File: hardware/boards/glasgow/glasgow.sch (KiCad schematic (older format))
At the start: 93 parts, among them J1 USB_B_Micro, U1 CY7C68013A-56LTX, U15 TPD3S014, U2 CAT24M01W, U3 CAT24C256W, U30 ICE40HX8K-BG121, U34 ATECC508A, U36 TLV73312PQDRVRQ1, U7 LM3880MF-1AF, U8 TLV75533PDRVR, Y1 24M

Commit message: revC2: added output files
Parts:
- removed J1: USB_B_Micro, Connector_USB:USB_Micro-B_Molex_47346-0001, symbol Connector:USB_B_Micro
- added J1: USB_C_Plug_USB2.0, Glasgow:USB-C_16Pin, symbol Connector:USB_C_Plug_USB2.0
- added R52, R53: 5k1, Resistor_SMD:R_0402_1005Metric, symbol Device:R
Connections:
- wire segments 364 -> 371
- no-connect marks 8 -> 7
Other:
- moved on the sheet: C13, FB1, R1, R2, R3, TP13, TP14, TP15, TP16, TP4, TP5

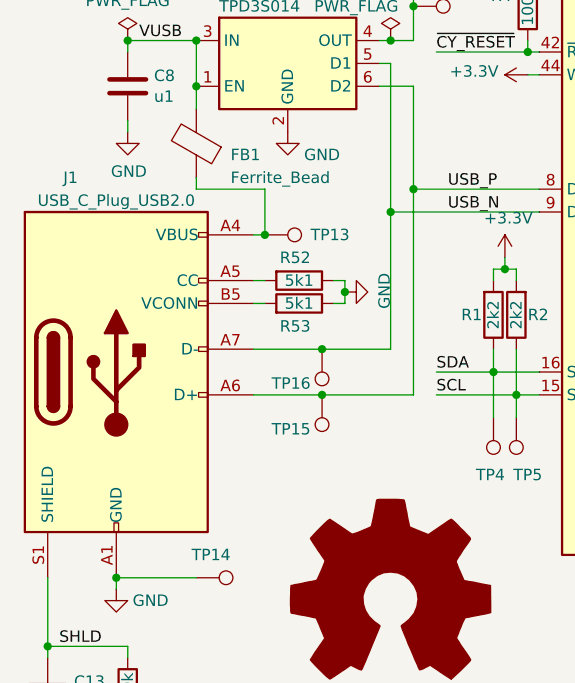
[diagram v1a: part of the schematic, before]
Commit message: added revC1 otter edition gerber
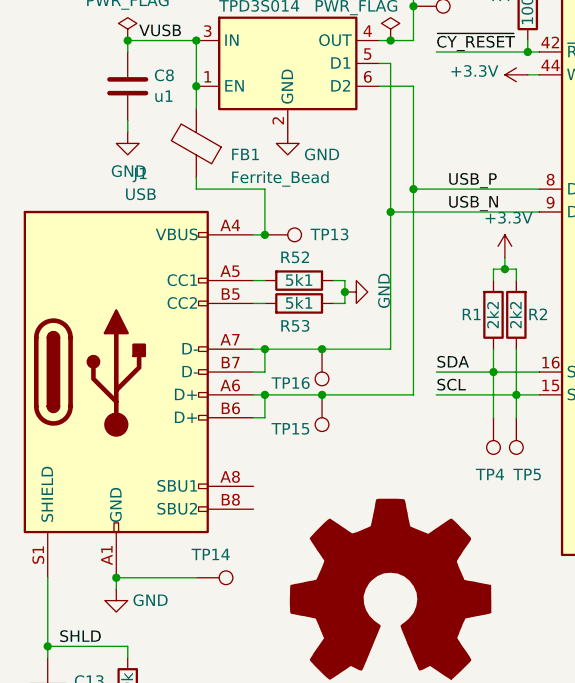
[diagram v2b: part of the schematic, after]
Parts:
- removed J1: USB_C_Plug_USB2.0, Glasgow:USB-C_16Pin, symbol Connector:USB_C_Plug_USB2.0
- added J1: USB, otter:USB-C 16Pin, symbol Connector:USB_C_Receptacle_USB2.0
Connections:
- net GND: now also J1.A1 (GND), J1.A12 (GND), J1.B1 (GND), J1.B12 (GND)
- net SHLD: now also J1.S1 (SHIELD)
- net USB_N: now also J1.A7 (D-), J1.B7 (D-)
- net USB_P: now also J1.A6 (D+), J1.B6 (D+)
- net at FB1.1, TP13.1: now also J1.A4 (VBUS), J1.A9 (VBUS), J1.B4 (VBUS), J1.B9 (VBUS)
- net at R52.2: now also J1.A5 (CC1)
- net at R53.2: now also J1.B5 (CC2)
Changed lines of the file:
@@
 	1050 3500 1350 3500
 Wire Wire Line
-	1600 4850 1900 4850
+	1600 4850 1650 4850
 Wire Wire Line
 	4950 6750 4950 6850
@@
 Text Notes 4550 7750 0    50   ~ 0
 Plug in the device while shorting R40 if it stops enumerating
-$Comp
-L Connector:USB_C_Plug_USB2.0 J1
-U 1 1 5E1816D0
-P 1000 4950
-F 0 "J1" H 800 5800 50  0000 C CNN
-F 1 "USB_C_Plug_USB2.0" H 1000 5700 50  0000 C CNN
-F 2 "Glasgow:USB-C_16Pin" H 1150 4950 50  0001 C CNN
-F 3 "https://www.usb.org/sites/default/files/USB%20Type-C%20Spec%20R2.0%20-%20August%202019.pdf" H 1150 4950 50  0001 C CNN
-F 4 "USB4105-GF-A " H 1000 4950 50  0001 C CNN "MPN"
-F 5 "GCT" H 1000 4950 50  0001 C CNN "Mfg"
-F 6 "" H 1000 4950 50  0001 C CNN "1b2-bom-key"
-	1    1000 4950
-	1    0    0    -1
-$EndComp
-Connection ~ 1000 5850
 Wire Wire Line
 	2400 5050 2750 5050
@@
 $EndComp
 Wire Wire Line
-	1600 5050 1900 5050
+	1600 5050 1650 5050
 $Comp
 L Device:R R52
@@
 Wire Wire Line
 	700  6150 1050 6150
+$Comp
+L Connector:USB_C_Receptacle_USB2.0 J1
+U 1 1 5E62D70A
+P 1000 4950
+F 0 "J1" H 1107 5817 50  0000 C CNN
+F 1 "USB" H 1107 5726 50  0000 C CNN
+F 2 "otter:USB-C 16Pin" H 1150 4950 50  0001 C CNN
+F 3 "https://www.usb.org/sites/default/files/documents/usb_type-c.zip" H 1150 4950 50  0001 C CNN
+	1    1000 4950
+	1    0    0    -1
+$EndComp
+Wire Wire Line
+	1600 5150 1650 5150
+Wire Wire Line
+	1650 5150 1650 5050
+Connection ~ 1650 5050
+Wire Wire Line
+	1650 5050 1900 5050
+Wire Wire Line
+	1600 4950 1650 4950
+Wire Wire Line
+	1650 4950 1650 4850
+Connection ~ 1650 4850
+Wire Wire Line
+	1650 4850 1900 4850
+Connection ~ 1000 5850
 Wire Bus Line
 	4700 6250 7850 6250
